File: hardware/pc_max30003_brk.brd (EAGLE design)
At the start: 32 x 26 mm, 32 parts, among them U2 TXB0108PWR, U4 AP2112K-3.3V

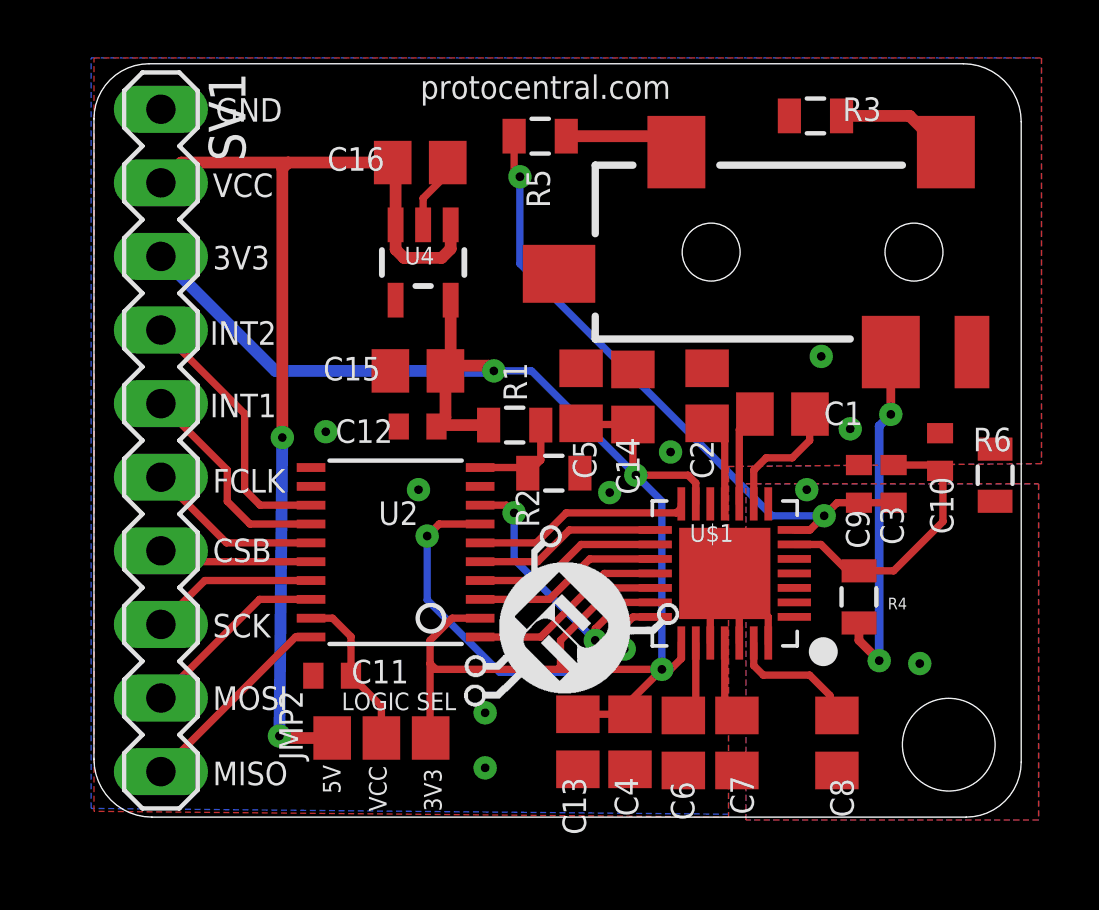
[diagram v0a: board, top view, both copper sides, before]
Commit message: updated design file
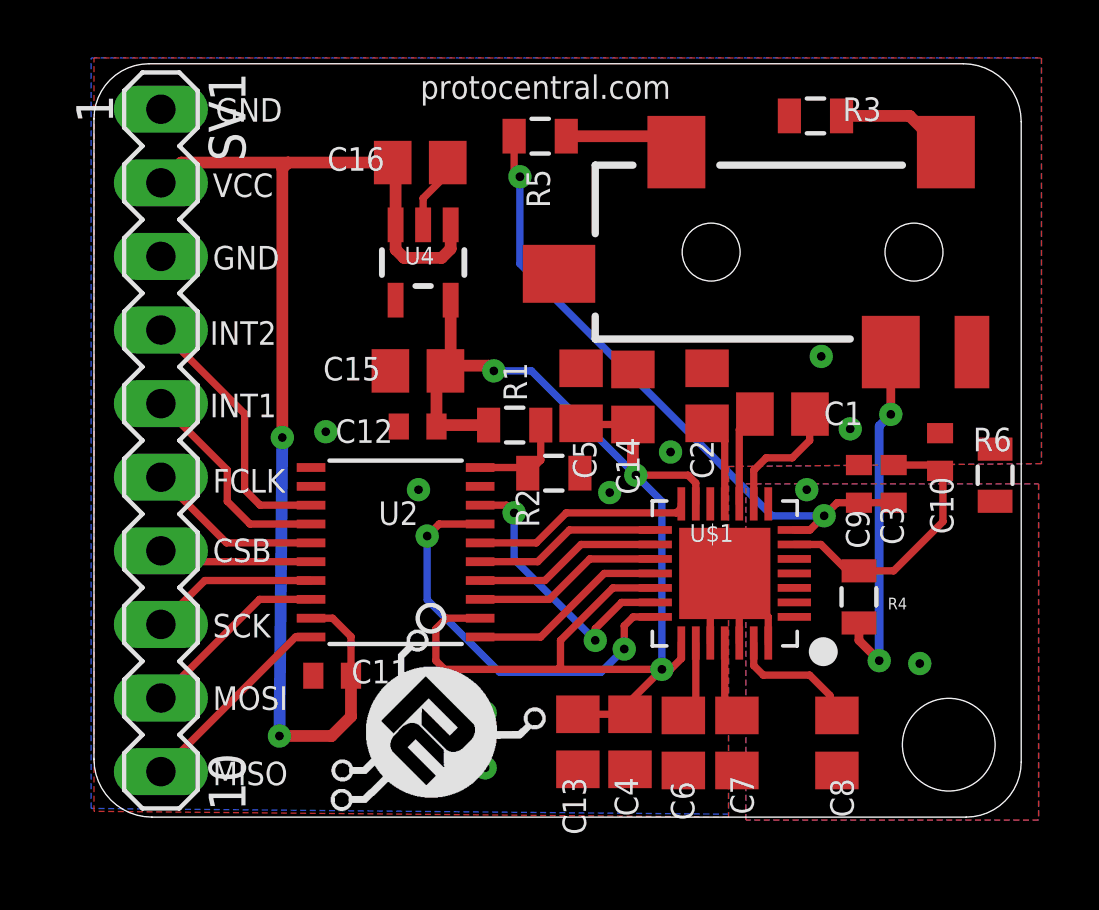
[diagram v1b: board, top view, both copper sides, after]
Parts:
- removed JMP2: 0R-JUMPA, jump-0r-smd:A0R-JMP
- U4: value AP2112K-3.3V -> AP2112K-1.8V
- moved U$6 20.6 mm to (28.7, 15.8)
- moved U$2 9.80 mm to (28.7, 4.80)
- moved U$7 7.22 mm to (19.3, 13.9)
- moved U$3 5.84 mm to (8.10, 0.10)
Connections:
- removed net +3V3: C12.2, C13.1, C14.1, C15.2, C4.1, C5.1, JMP2.3, R1.1, SV1.3, U$1.13, U$1.19, U$1.22, U2.2, U4.5
- removed net VCC: C11.2, JMP2.2, U2.19
- new net +1.8V: C12.2, C13.1, C14.1, C15.2, C4.1, C5.1, R1.1, U$1.13, U$1.19, U$1.22, U2.2, U4.5
- net GND: now also SV1.3
- net VDD: now also C11.2, U2.19; no longer JMP2.1
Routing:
- net +3V3: track 64.8 -> 0.00 mm, vias 3 -> 0
- net +1.8V: track 0.00 -> 48.8 mm, vias 0 -> 3
- net VCC: track 5.58 -> 0.00 mm
- net VDD: track 36.0 -> 41.3 mm
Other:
- board text added: "VCC: 3.3 to 5V Logic: 3.3 to 5V"
- board text added: "v1.1"
- board text removed: "3V3"
- board text removed: "5V"
- board text removed: "LOGIC SEL"
